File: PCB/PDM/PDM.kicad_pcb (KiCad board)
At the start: 2 copper layers, 133 parts, among them IC1 BTS70021EPPXUMA1, IC10 BTS70021EPPXUMA1, IC11 BTS70021EPPXUMA1, IC12 LM5050MK-1_NOPB, IC13 LM5050MK-1_NOPB, IC2 BTS70021EPPXUMA1, IC3 BTS500101TAEATMA1, IC4 TS5A21366DCUR, IC5 TMP126NDCKR, IC6 TMP126NDCKR, IC7 BTS722204ESAXUMA1, IC8 BTS722204ESAXUMA1, IC9 BTS500101TAEATMA1, Q1 MMBT3904, Q2 IAUA250N04S6N007AUMA1, Q3 IAUA250N04S6N007AUMA1, U1 STM32F405RGTx, U2 MCP2561-E-SN, U3 MCP2561-E-SN

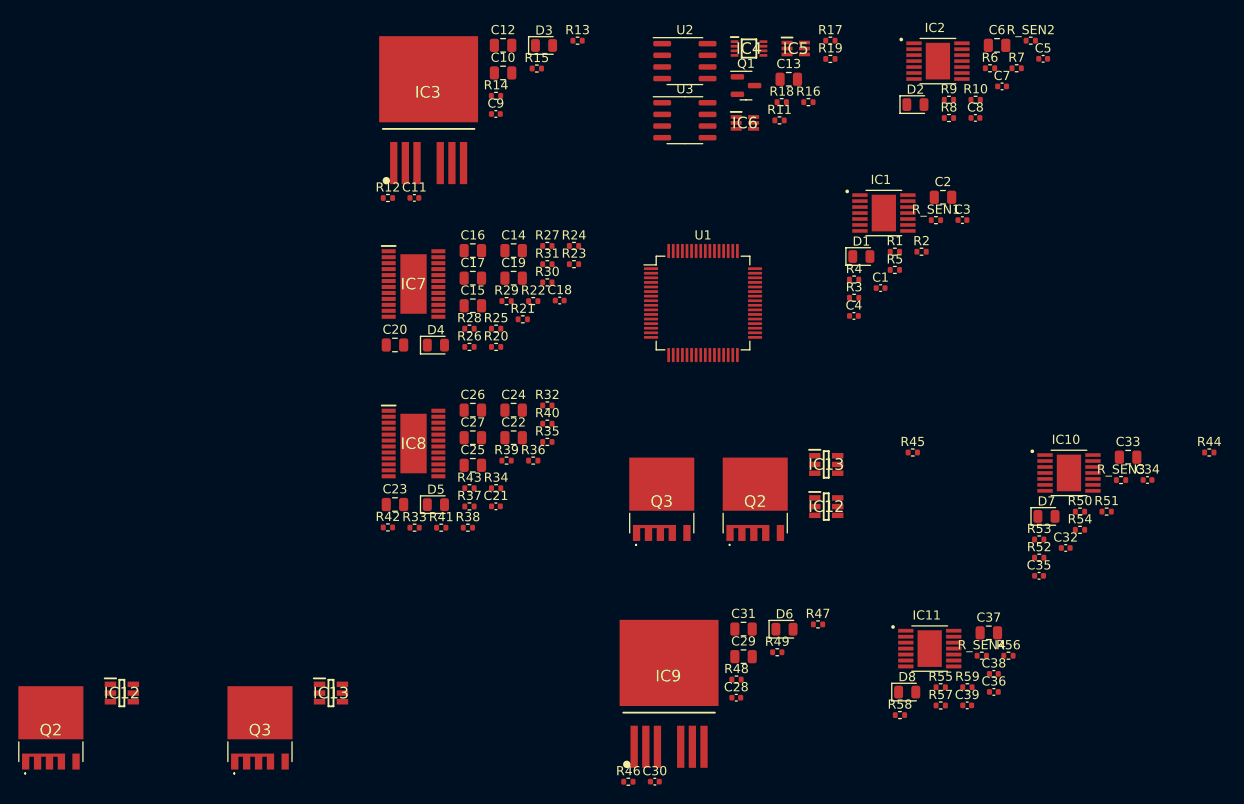
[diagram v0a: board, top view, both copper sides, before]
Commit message: Fuck christmas & low side section
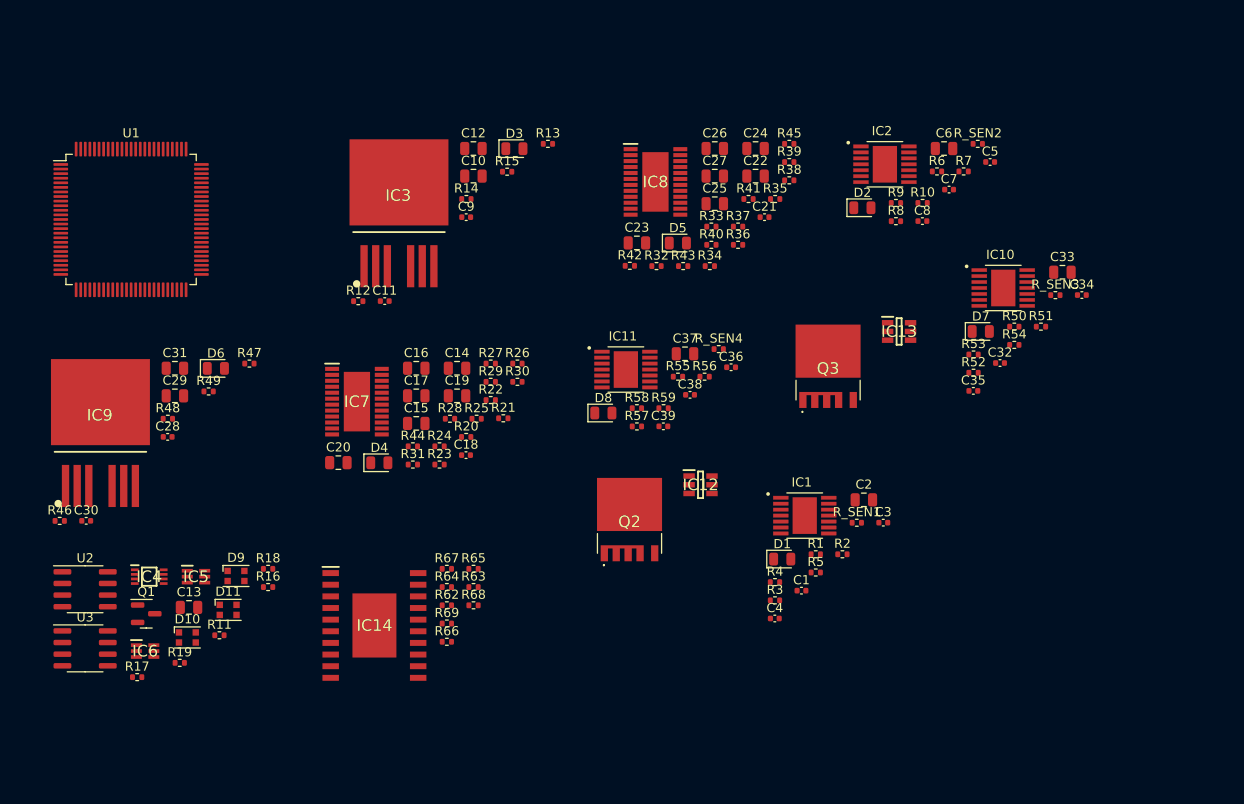
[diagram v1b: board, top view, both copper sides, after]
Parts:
- removed the IC12 at (172.7, 90.9)
- removed the IC12 at (249.6, 70.6)
- removed the IC13 at (249.6, 66.0)
- removed the IC13 at (195.5, 90.9)
- removed the Q2 at (241.8, 71.0)
- removed the Q2 at (165.0, 96.0)
- removed the Q3 at (231.6, 71.0)
- removed the Q3 at (187.8, 96.0)
- added D10: WS2812B, LED_SMD:LED_WS2812B-2020_PLCC4_2.0x2.0mm, F.Cu at (179.9, 84.9)
- added D11: WS2812B, LED_SMD:LED_WS2812B-2020_PLCC4_2.0x2.0mm, F.Cu at (184.3, 81.9)
- added D9: WS2812B, LED_SMD:LED_WS2812B-2020_PLCC4_2.0x2.0mm, F.Cu at (185.2, 78.2)
- added IC12: LM5050MK-1_NOPB, PDM_Additional:SOT95P280X110-6N, F.Cu at (235.9, 68.2)
- added IC13: LM5050MK-1_NOPB, PDM_Additional:SOT95P280X110-6N, F.Cu at (257.5, 51.5)
- added IC14: TLE8104E, PDM_Additional:SOIC127P1030X255-21N, F.Cu at (200.3, 83.6)
- added Q2: IAUA250N04S6N007AUMA1, PDM_Additional:IAUA250N04S6N007AUMA1, F.Cu at (228.1, 73.3)
- added Q3: IAUA250N04S6N007AUMA1, PDM_Additional:IAUA250N04S6N007AUMA1, F.Cu at (249.8, 56.5)
- added R62: 1.2k, Resistor_SMD:R_0402_1005Metric, F.Cu at (208.2, 81.4)
- added R63: 4.7k, Resistor_SMD:R_0402_1005Metric, F.Cu at (211.1, 79.4)
- added R64: 4.7k, Resistor_SMD:R_0402_1005Metric, F.Cu at (208.2, 79.4)
- added R65: 4.7k, Resistor_SMD:R_0402_1005Metric, F.Cu at (211.1, 77.4)
- added R66: 4.7k, Resistor_SMD:R_0402_1005Metric, F.Cu at (208.2, 85.3)
- added R67: 1.2k, Resistor_SMD:R_0402_1005Metric, F.Cu at (208.2, 77.4)
- added R68: 1.2k, Resistor_SMD:R_0402_1005Metric, F.Cu at (211.1, 81.4)
- added R69: 1.2k, Resistor_SMD:R_0402_1005Metric, F.Cu at (208.2, 83.3)
- U1: value STM32F405RGTx -> STM32L496VGTx; footprint Package_QFP:LQFP-64_10x10mm_P0.5mm -> Package_QFP:LQFP-100_14x14mm_P0.5mm
- moved R17 102.7 mm to (174.4, 89.2)
- moved R19 96.9 mm to (179.0, 87.6)
- moved Q1 87.2 mm to (175.4, 82.3)
- moved IC5 87.2 mm to (180.8, 78.2)
- moved C13 87.2 mm to (180.0, 81.6)
- moved IC6 87.2 mm to (175.3, 86.4)
- moved U3 87.2 mm to (168.7, 86.1)
- moved IC4 87.2 mm to (175.7, 78.2)
- moved U2 87.2 mm to (168.7, 79.6)
- moved R44 86.9 mm to (204.5, 64.0)
- moved R11 83.0 mm to (183.4, 84.6)
- moved R16 79.2 mm to (188.7, 79.4)
- moved R18 75.7 mm to (188.7, 77.4)
- moved C28 68.3 mm to (177.7, 63.0)
- moved R46 68.3 mm to (165.9, 72.1)
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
